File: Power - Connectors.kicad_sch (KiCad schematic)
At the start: 0 parts

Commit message: [01/07/2026][MCU - IOs] Update
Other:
- company: (none) -> ${COMPANY}
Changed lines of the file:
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@@
 	(generator_version "9.0")
 	(paper "A4")
+	(title_block
+		(date "2026-06-27")
+		(company "${COMPANY}")
+	)
 )

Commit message: Update Power Connector & Motor Control Schematic
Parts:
- added C44, C45, C46, C47: 0.1uF 35V 0603, Duc:C0603, symbol Duc-Capacitors:CAP CER 0603
- added J1: DC-044A-20A, Duc:DC-IN-TH_DC-044A-20A, symbol Duc-Connectors:DC-044A-20A
- added J1: XT60PW-M, Duc:CONN-TH_XT60PW-M, symbol Duc-Connectors:XT60PW-M
- added Q1, Q2: HV10N03, Duc:SOT-89-3_L4.5-W2.5-P1.50-LS4.0-BR, symbol Duc-Transistors:HV10N03
- added U8, U9: LM74700QDBVRQ1, Duc:SOT-23-6_L2.9-W1.6-P0.95-LS2.8-BL, symbol Duc-Power:LM74700QDBVRQ1
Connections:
- new net: C45.2, U8.1 (VCAP)
- new net: Q1.1 (G), U8.5 (GATE)
- new net: C47.2, U9.1 (VCAP)
- new net: Q2.1 (G), U9.5 (GATE)
- new net +VBAT: Q1.3 (S), Q2.3 (S), U8.4 (CATHODE), U9.4 (CATHODE)
- new net +V_ADAPTER: C46.1, C47.1, J1.1, Q2.2 (D), U9.3 (EN), U9.6 (ANODE)
- new net +V_BAT2S: C44.1, C45.1, J1.2 (+), Q1.2 (D), U8.3 (EN), U8.6 (ANODE)
- new net GND: C44.2, C46.2, J1.1 (-), J1.2, J1.3, U8.2 (GND), U9.2 (GND)
- no-connect marks 0 -> 4

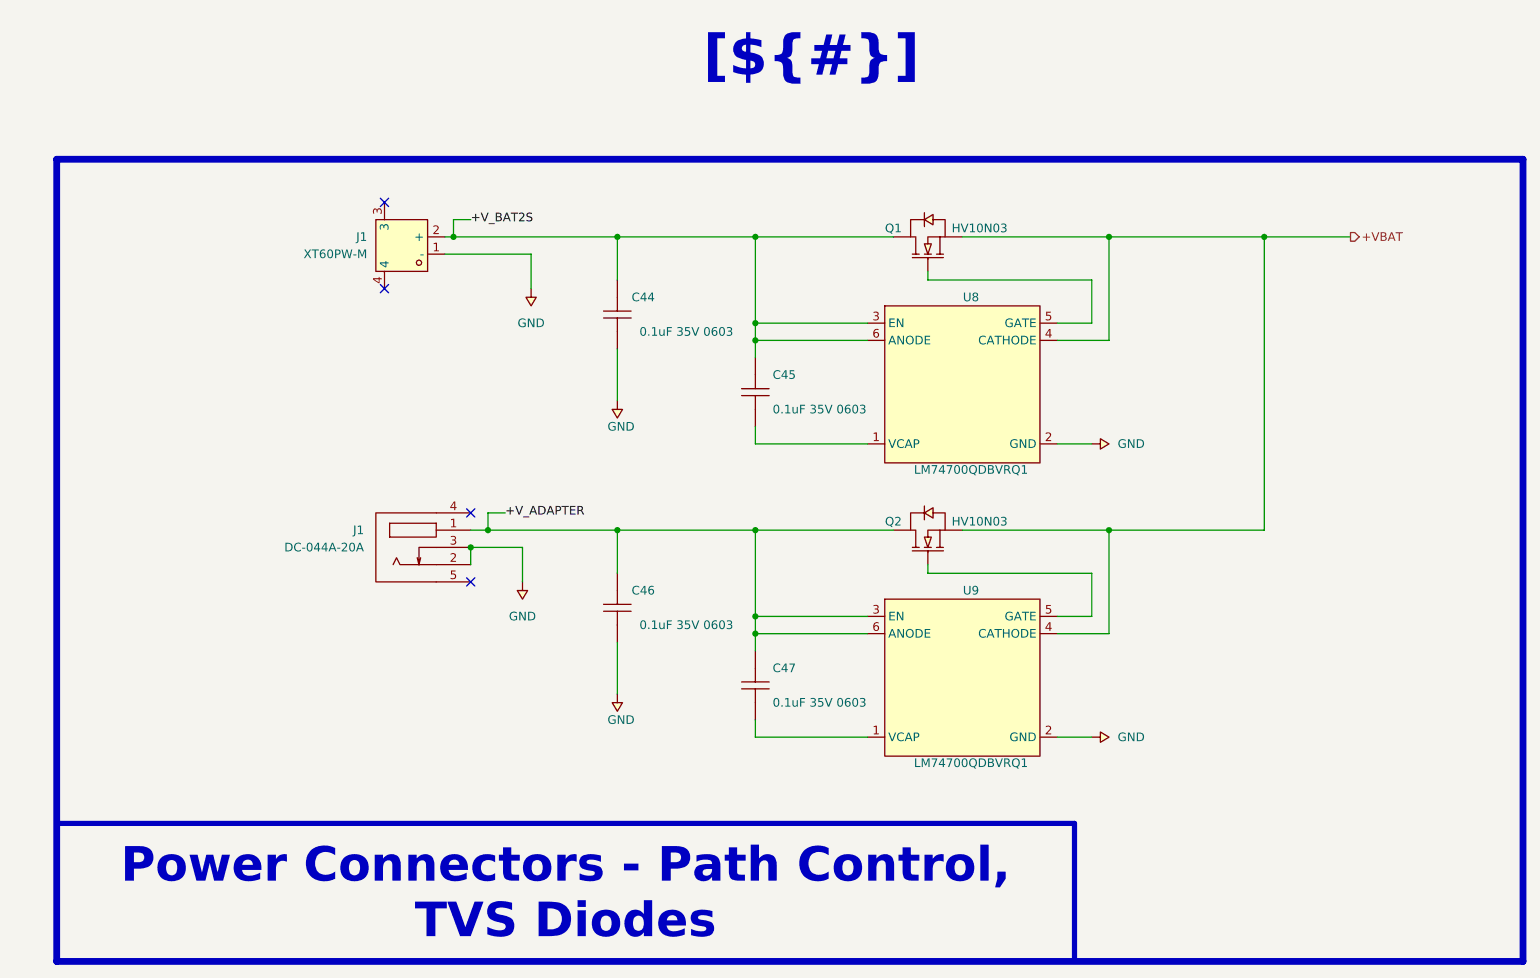
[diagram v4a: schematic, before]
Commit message: Update Schematic
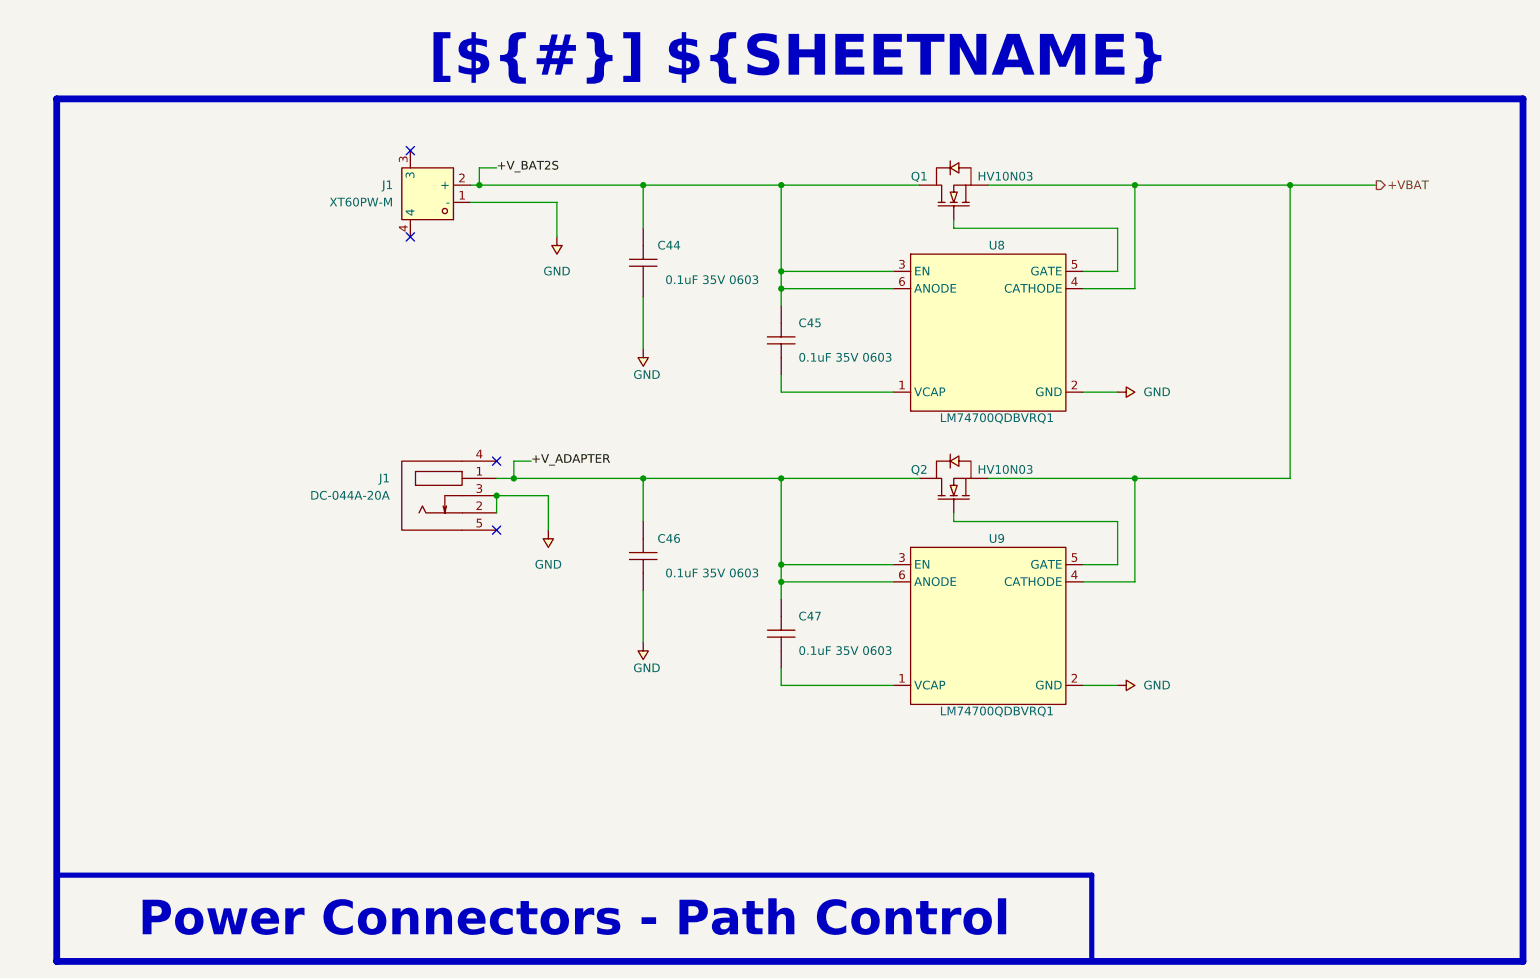
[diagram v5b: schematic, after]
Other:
- moved on the sheet: C44, C45, C46, C47, J1, Q1, Q2, U8, U9
